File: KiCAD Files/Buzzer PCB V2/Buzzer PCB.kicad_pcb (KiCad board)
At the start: 2 copper layers, 90 x 50 mm, 18 parts, among them J1 2600mAh LiPo JST-PH bottom, J10 Adafruit ESP32 Feather V2 hea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, J11 OLED FeatherWing header, J2 Legacy SW_BAT/GND out, J3 SD card module, swapped pins, J4 Legacy D13 test pad, J5 GPS M100 Mini, J6 BMP390/BMP5xx top module, J7 SHT41 top module, Q1 S8050, SW1 SS12D00G5, U1 TP4057 USB-C charger

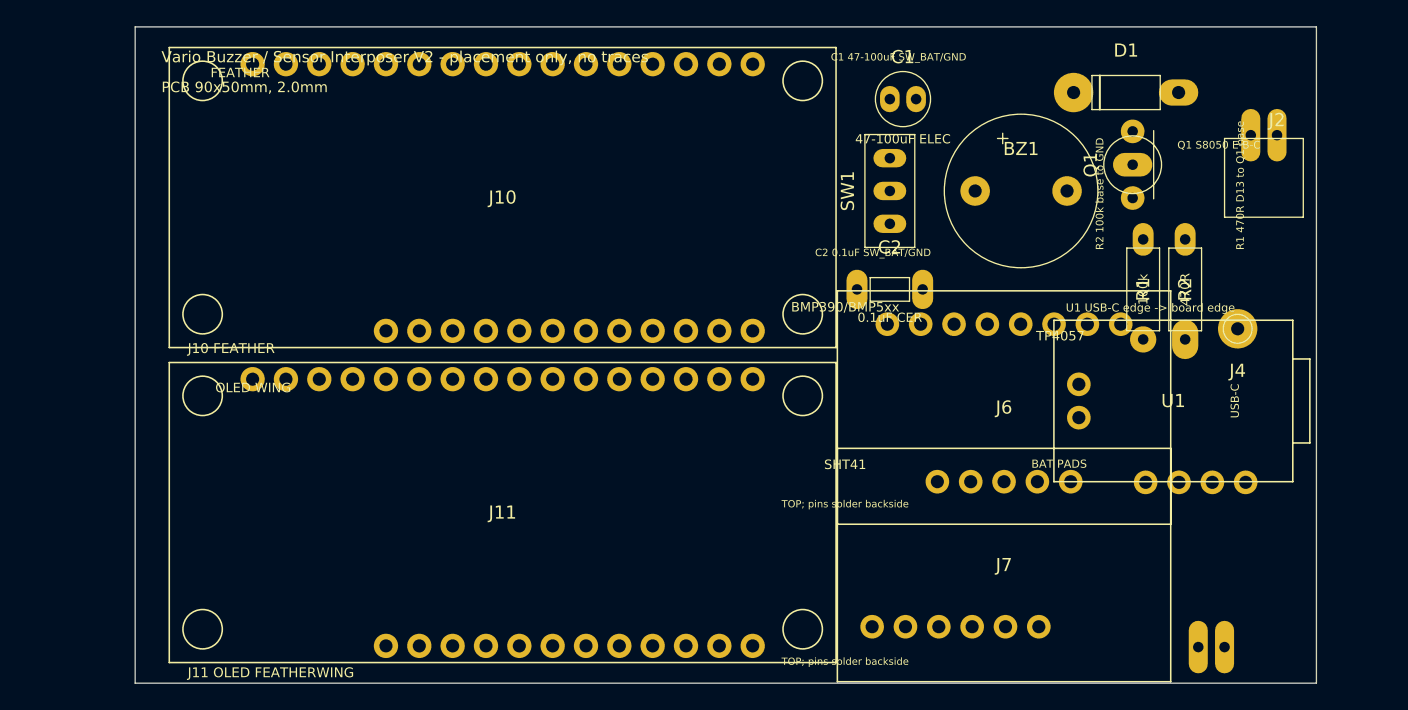
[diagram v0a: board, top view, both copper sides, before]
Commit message: V2 with sparkfun
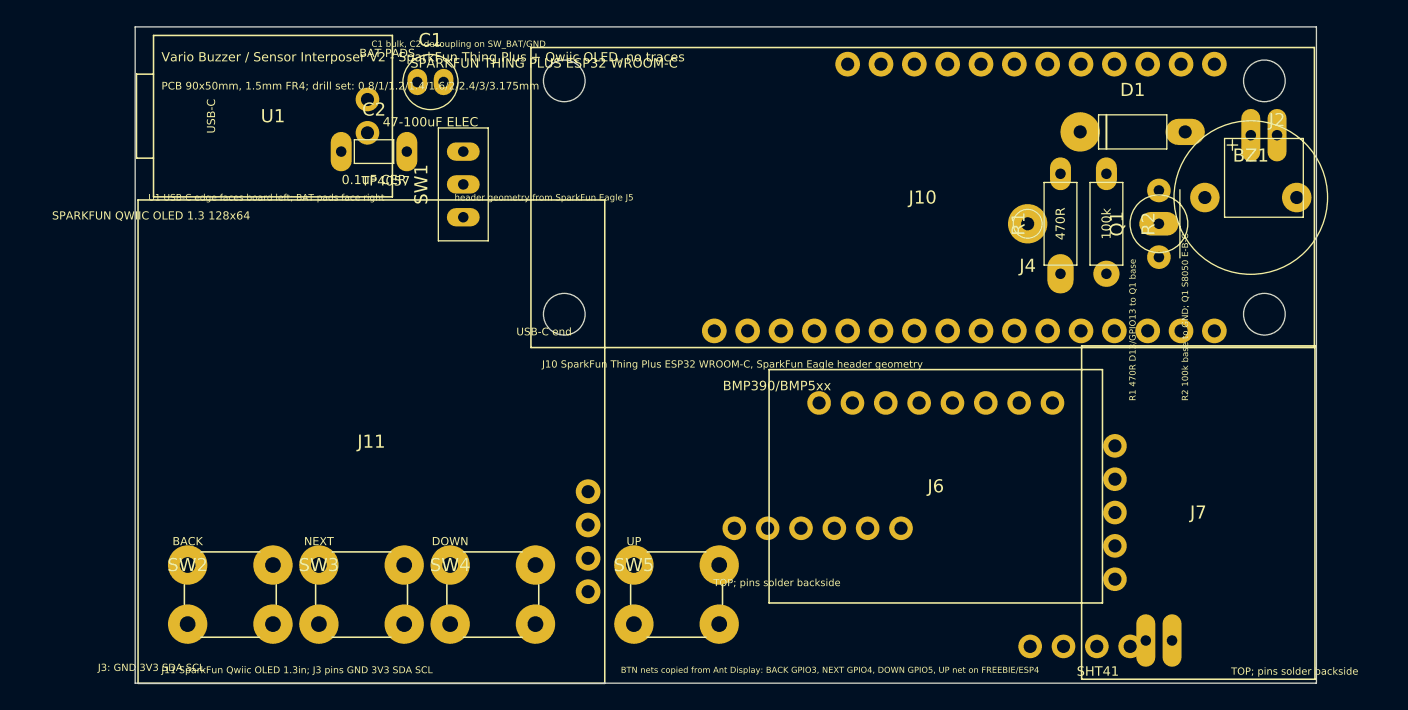
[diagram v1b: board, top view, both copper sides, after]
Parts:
- added SW2: BACK, Vario_Buzzer_V2:Ant_Display_SW_PUSH_6mm_H5mm, F.Cu at (4.00, 41.0)
- added SW3: NEXT, Vario_Buzzer_V2:Ant_Display_SW_PUSH_6mm_H5mm, F.Cu at (14.0, 41.0)
- added SW4: DOWN, Vario_Buzzer_V2:Ant_Display_SW_PUSH_6mm_H5mm, F.Cu at (24.0, 41.0)
- added SW5: UP, Vario_Buzzer_V2:Ant_Display_SW_PUSH_6mm_H5mm, F.Cu at (38.0, 41.0)
- J10: value Adafruit ESP32 Feather V2 header -> SparkFun Thing Plus ESP32 WROOM-C USB-C header; footprint Vario_Buzzer_V2:Feather_28_Header_Separate -> Vario_Buzzer_V2:SparkFun_Thing_Plus_ESP32_WROOM_C_Header
- J11: value OLED FeatherWing header -> SparkFun Qwiic OLED 1.3in module; footprint Vario_Buzzer_V2:OLED_FeatherWing_28_Header -> Vario_Buzzer_V2:SparkFun_Qwiic_OLED_1p3_Module
- J3: value SD card module, swapped pins -> Optional external SD module; Thing Plus has onboard microSD
- J5: value GPS M100 Mini -> HGLRC M100 Mini GPS manual pinout
- J6: value BMP390/BMP5xx top module -> BMP390/BMP5xx top pads
- J7: value SHT41 top module -> SHT41 top pads
- moved U1 72.0 mm to (10.5, 6.80), turned to 180 degrees
- moved C2 40.7 mm to (18.2, 9.50)
- moved C1 36.0 mm to (22.5, 4.20)
- moved SW1 32.5 mm to (25.0, 12.0)
- moved J10 32.0 mm to (60.0, 13.0)
- moved J4 17.9 mm to (68.0, 15.0)
- moved BZ1 17.5 mm to (85.0, 13.0)
- moved J7 15.3 mm to (81.0, 37.0), turned to 90 degrees
- moved J5 15.3 mm to (72.0, 41.5)
- moved J3 12.9 mm to (52.0, 31.0)
- moved J11 11.4 mm to (18.0, 31.6)
- moved R1 10.7 mm to (70.5, 15.0)
- moved J6 7.94 mm to (61.0, 35.0)
- moved R2 5.73 mm to (74.0, 15.0)
- moved Q1 4.92 mm to (78.0, 15.0)
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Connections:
- J10 pad 1: RESET -> SDA
- J10 pad 11: SPI_SCK -> (no net)
- J10 pad 12: SPI_MOSI -> SW_BAT
- J10 pad 13: SPI_MISO -> BTN_UP_GPIO21
- J10 pad 14: GPS_TX_FEATHER_RX -> GPS_RX_THING_TX
- J10 pad 15: GPS_RX_FEATHER_TX -> GPS_TX_THING_RX
- J10 pad 16: (no net) -> SPI_MISO
- J10 pad 17: SDA -> SPI_MOSI
- J10 pad 18: SCL -> SPI_SCK
- J10 pad 19: D5_IO14_BTN_C -> (no net)
- J10 pad 2: 3V3 -> SCL
- J10 pad 20: D6_IO32_BTN_B -> (no net)
- J10 pad 21: D9_IO15_BTN_A -> (no net)
- J10 pad 22: SD_CS_D10_IO27 -> (no net)
- J10 pad 25: D13 -> GND
- J10 pad 27: (no net) -> 3V3
- J10 pad 28: SW_BAT -> (no net)
- J10 pad 4: GND -> BTN_DOWN_GPIO5
- J10 pad 5: (no net) -> BTN_NEXT_GPIO4
- J10 pad 6: (no net) -> BTN_BACK_GPIO3
- J10 pad 7: (no net) -> SD_CS_GPIO2
- J10 pad 9: (no net) -> D13_BUZZER_GPIO13
- J11 pad 1: RESET -> GND
- J11 pad 3: (no net) -> SDA
- J11 pad 4: GND -> SCL
- J3 pad 5: SD_CS_D10_IO27 -> SD_CS_GPIO2
- J4 pad e: D13 -> D13_BUZZER_GPIO13
- J5 pad 1: GND -> GPS_RX_THING_TX
- J5 pad 2: 3V3 -> GPS_TX_THING_RX
- J5 pad 3: GPS_TX_FEATHER_RX -> 3V3
- J5 pad 4: GPS_RX_FEATHER_TX -> GND
- R1 pad 1: D13 -> D13_BUZZER_GPIO13
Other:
- board text added: "BTN nets copied from Ant Display: BACK GPIO3, NEXT GPIO4, DOWN GPIO5, UP net on FREEBIE/ESP4"
- board text added: "Back side: optional external SD plus HGLRC M100"
- board text added: "C1 bulk, C2 decoupling on SW_BAT/GND"
- board text added: "J1 bottom LiPo JST"
- board text added: "J10 SparkFun Thing Plus ESP32 WROOM-C, SparkFun Eagle header geometry"
- board text added: "J11 SparkFun Qwiic OLED 1.3in; J3 pins GND 3V3 SDA SCL"
- board text added: "J5 HGLRC M100 manual pin order: RX TX VCC GND"
- board text added: "PCB 90x50mm, 1.5mm FR4; drill set: 0.8/1/1.2/1.4/1.6/2/2.4/3/3.175mm"
- board text added: "R1 470R D13/GPIO13 to Q1 base"
- board text added: "R2 100k base to GND; Q1 S8050 E-B-C"
- board text added: "U1 USB-C edge faces board left; BAT pads face right"
- board text added: "Vario Buzzer / Sensor Interposer V2 - SparkFun Thing Plus + Qwiic OLED, no traces"
- board text removed: "Back: SD + M100"
- board text removed: "C1 47-100uF SW_BAT/GND"
- board text removed: "C2 0.1uF SW_BAT/GND"
- board text removed: "J1 bottom: LiPo JST"
- board text removed: "J10 FEATHER"
- board text removed: "J11 OLED FEATHERWING"
- board text removed: "PCB 90x50mm, 2.0mm"
- board text removed: "Q1 S8050 E-B-C"
- board text removed: "R1 470R D13 to Q1 base"
- board text removed: "R2 100k base to GND"
- board text removed: "U1 USB-C edge -> board edge"
- board text removed: "Vario Buzzer / Sensor Interposer V2 - placement only, no traces"
